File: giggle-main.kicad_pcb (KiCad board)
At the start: 2 copper layers, 97.5 x 97 mm, 27 parts, among them J1 CONN_05X2SHD, J2 CONN_05X2SHD

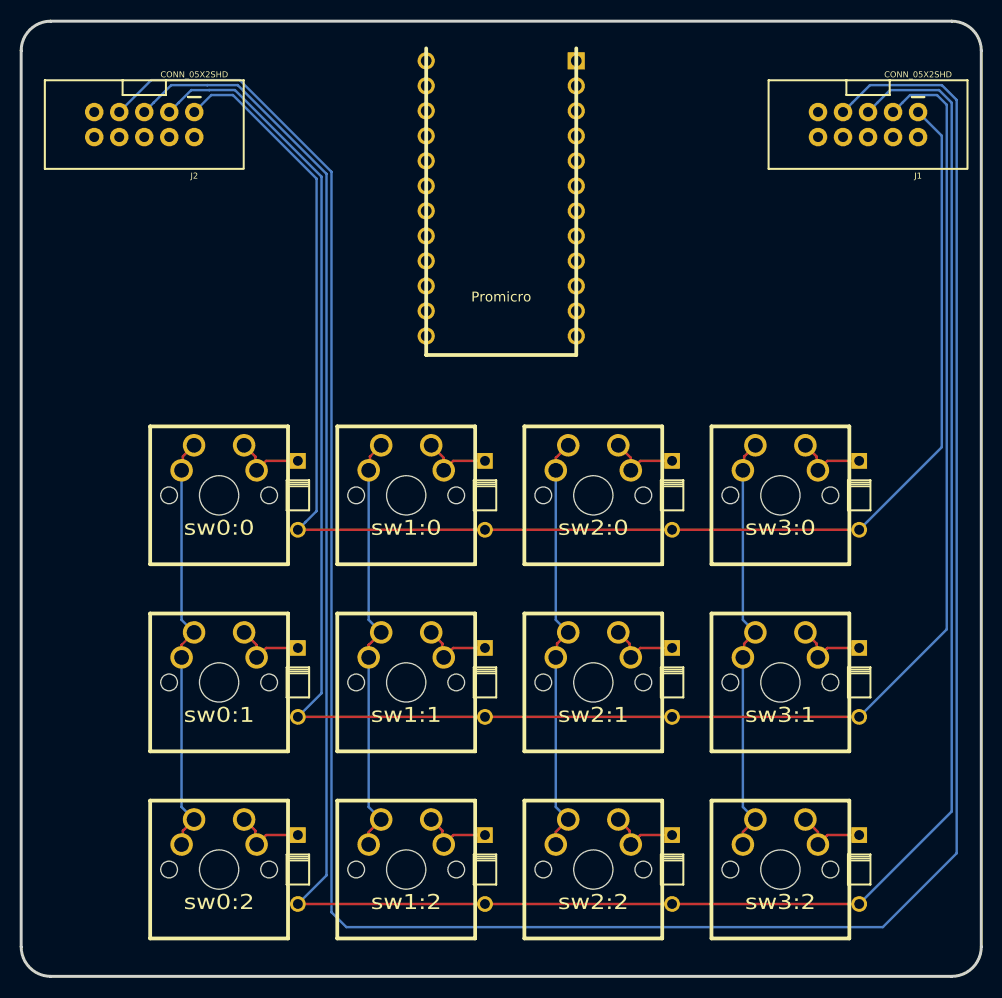
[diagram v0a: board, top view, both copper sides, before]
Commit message: finished main side.
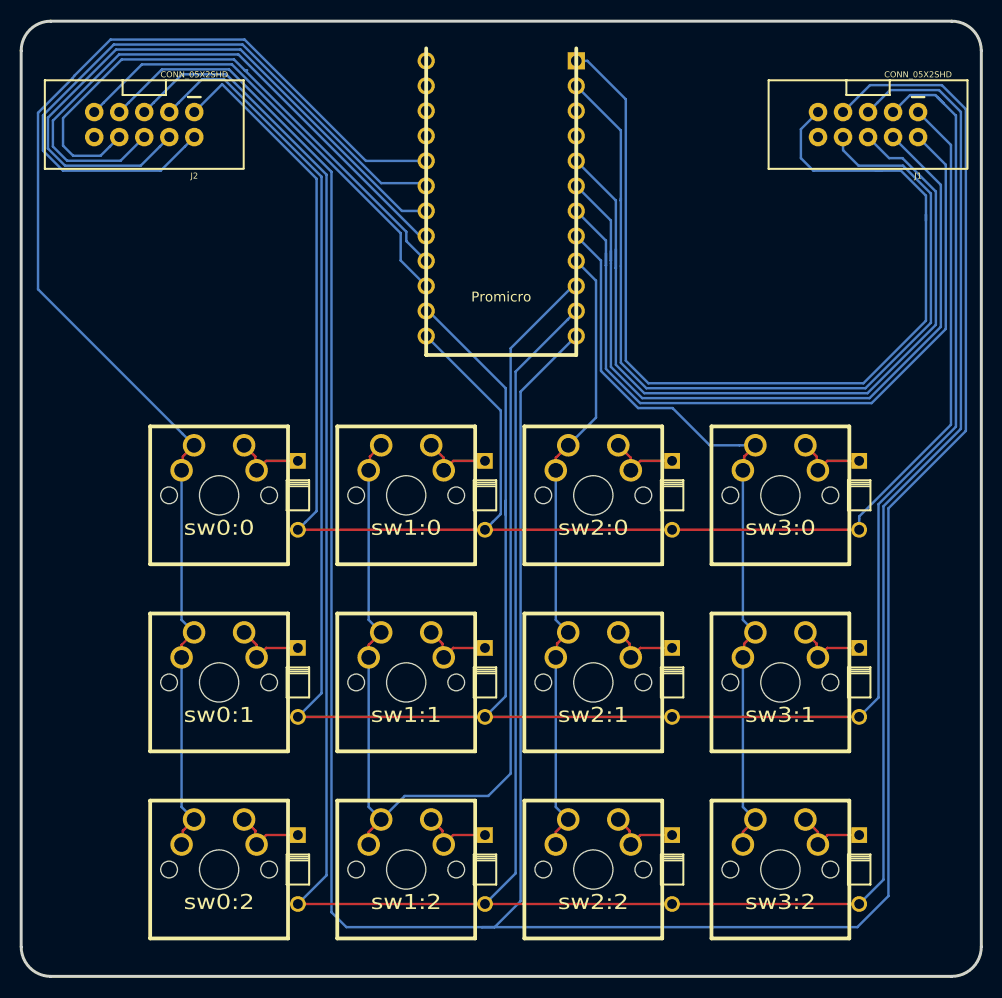
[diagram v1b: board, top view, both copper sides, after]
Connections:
- Promicro pad B1: (no net) -> N-col-0
- Promicro pad B2: (no net) -> N-row-1
- Promicro pad B3: (no net) -> N-col-4
- Promicro pad B4: (no net) -> N-row-2
- Promicro pad B5: (no net) -> N-row-3
- Promicro pad B6: (no net) -> N-row-0
- Promicro pad C6: (no net) -> N-col-8
- Promicro pad D0: (no net) -> N-col-11
- Promicro pad D1: (no net) -> N-col-10
- Promicro pad D4: (no net) -> N-col-12
- Promicro pad D7: (no net) -> N-col-7
- Promicro pad E6: (no net) -> N-col-6
- Promicro pad F4: (no net) -> N-col-5
- Promicro pad F5: (no net) -> N-col-3
- Promicro pad F6: (no net) -> N-col-2
- Promicro pad F7: (no net) -> N-col-1
- Promicro pad RX1: (no net) -> N-col-9
- Promicro pad TX0: (no net) -> N-col-13
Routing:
- net N-col-13: track 0.00 -> 100.8 mm
- net N-col-9: track 0.00 -> 90.7 mm
- net N-col-5: track 43.2 -> 131.1 mm
- net N-col-10: track 0.00 -> 83.6 mm
- net N-col-11: track 0.00 -> 79.9 mm
- net N-col-12: track 0.00 -> 78.3 mm
- net N-col-3: track 0.00 -> 69.0 mm
- net N-col-6: track 43.2 -> 110.7 mm
- net N-row-2: track 250.9 -> 316.6 mm
- net N-col-2: track 0.00 -> 65.5 mm
- net N-row-3: track 259.0 -> 323.9 mm
- net N-col-1: track 0.00 -> 61.2 mm
- net N-col-0: track 0.00 -> 58.3 mm
- net N-row-1: track 205.3 -> 254.6 mm
- net N-col-4: track 0.00 -> 46.7 mm
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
